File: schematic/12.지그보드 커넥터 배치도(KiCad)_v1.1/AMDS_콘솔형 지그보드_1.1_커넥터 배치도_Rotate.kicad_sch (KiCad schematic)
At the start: 37 parts, among them J1 Fan1, J1C01 POWER, J1C03 TEMP, J1C04 LED_DP1, J1C05 LED_DP2, J1C06 LED_TEMP, J1C07 LED_PSU, J1C08 LED_FAN#1, J1C09 LED_FAN#2, J1C10 DP_USB_SW, J1C15 DP, J1C18 PSU, J1C2 FAN, J2 Fan1, J3 Fan1, J4 Fan1, J5 Fan1, J6 Fan1, P1 Fan1, P2 Fan2, P3 Fan3, P4 Fan4, P5 Fan5, P6 Fan6

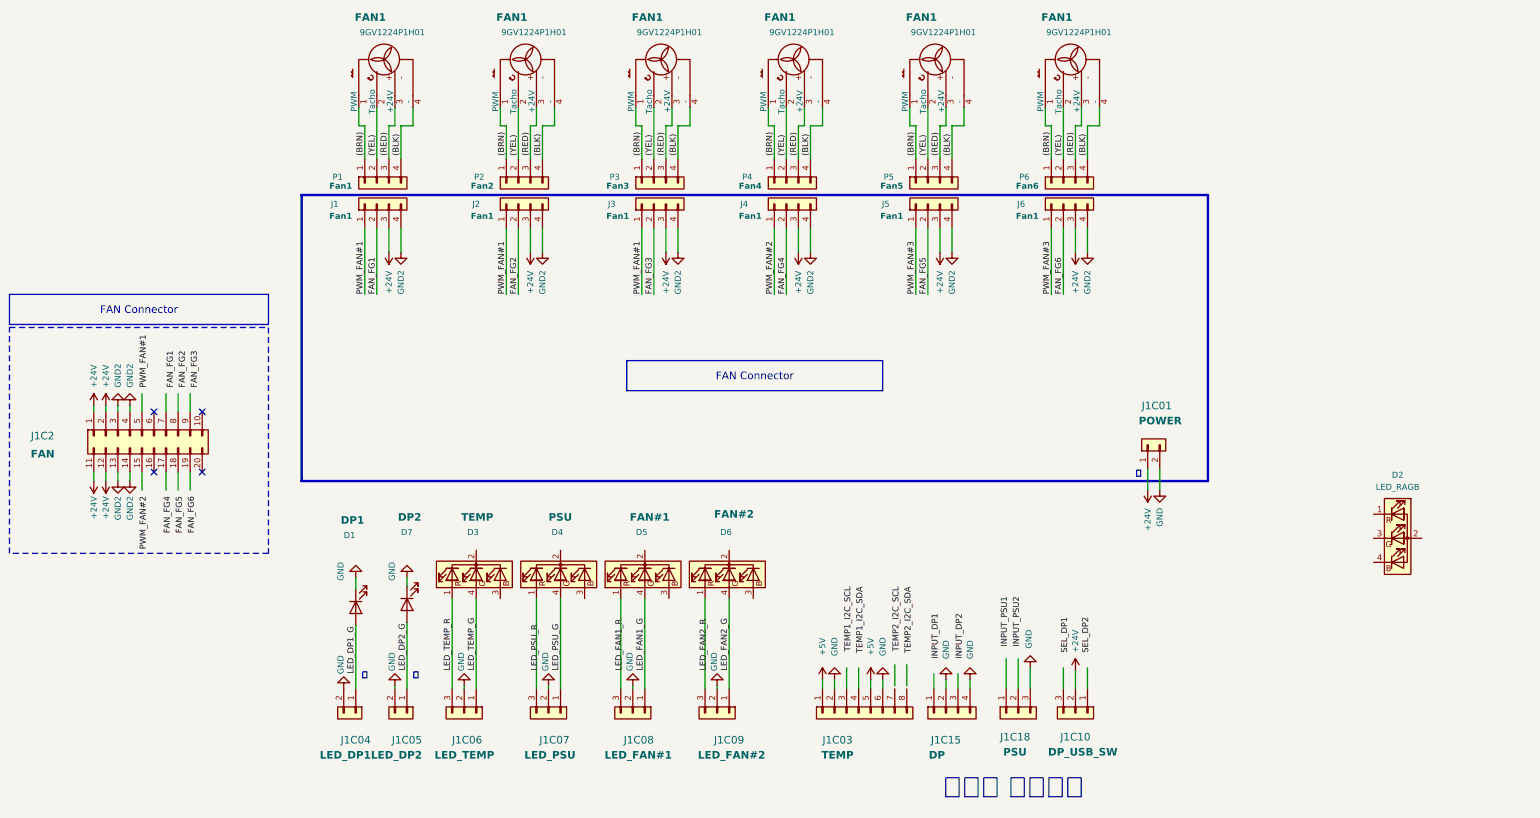
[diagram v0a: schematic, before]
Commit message: 24.12.20B
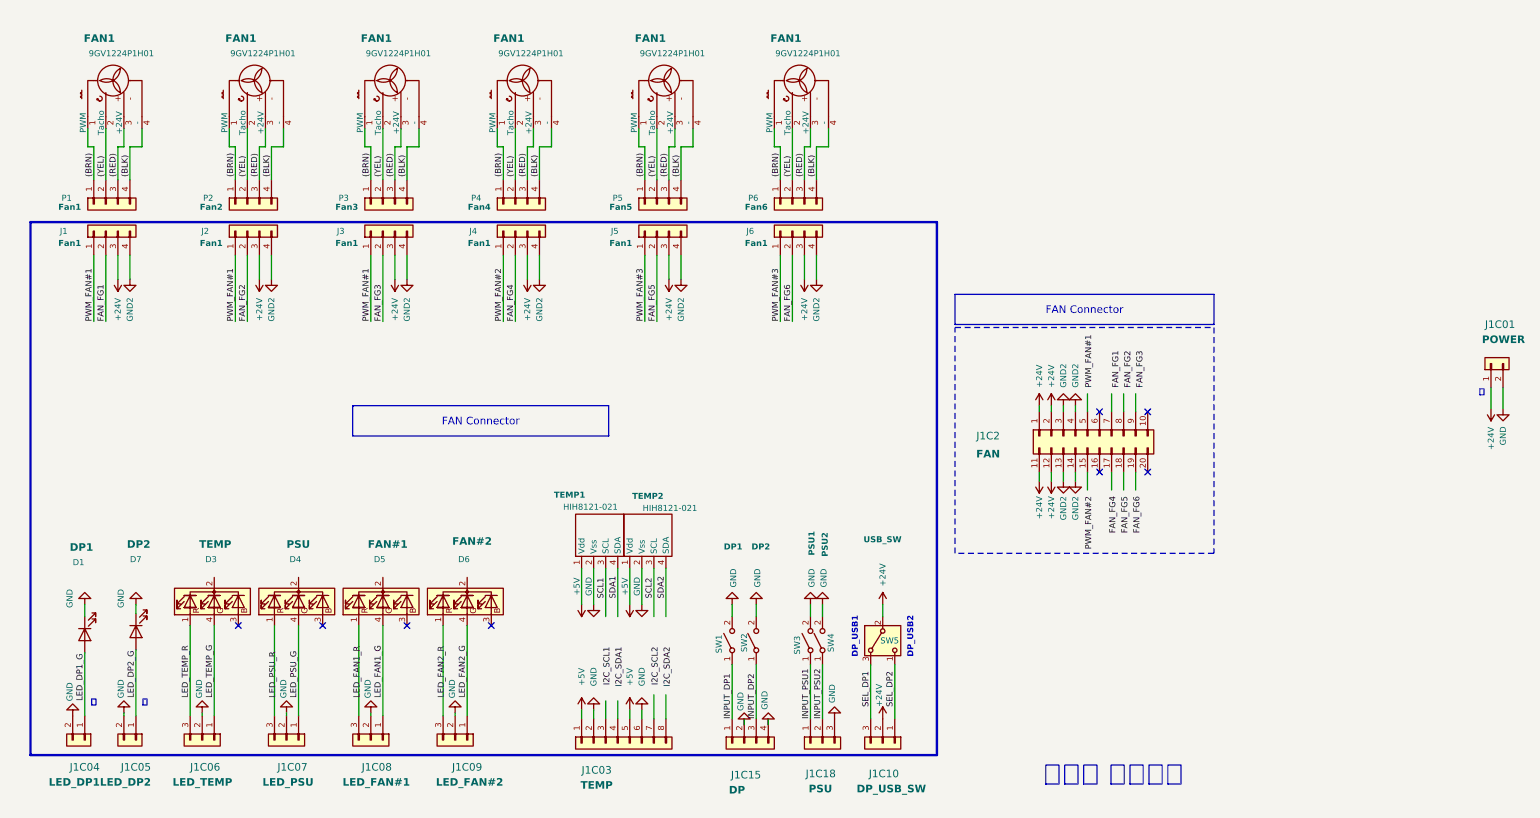
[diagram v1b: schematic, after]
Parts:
- removed D2: LED_RAGB, symbol Device:LED_RAGB
- added SW1: DP1, symbol Switch:SW_SPST
- added SW2: DP2, symbol Switch:SW_SPST
- added SW3: PSU1, symbol Switch:SW_SPST
- added SW4: PSU2, symbol Switch:SW_SPST
- added SW5: USB_SW, symbol Switch:SW_SPDT_321
- added TEMP1, TEMP2: HIH8121-021, symbol Graphic:HIH8121-021
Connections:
- net +24V: now also SW5.2 (B)
- net +5V: now also TEMP1.1 (Vdd), TEMP2.1 (Vdd)
- net GND: now also SW1.2 (B), SW2.2 (B), SW3.2 (B), SW4.2 (B), TEMP1.2 (Vss), TEMP2.2 (Vss)
- net INPUT_DP1: now also J1C15.1 (Pin_1), SW1.1 (A)
- net INPUT_DP2: now also J1C15.3 (Pin_3), SW2.1 (A)
- net INPUT_PSU1: now also J1C18.1 (Pin_1), SW3.1 (A)
- net INPUT_PSU2: now also J1C18.2 (Pin_2), SW4.1 (A)
- net SEL_DP1: now also J1C10.3 (Pin_3), SW5.3 (A)
- net SEL_DP2: now also J1C10.1 (Pin_1), SW5.1 (C)
- new net SCL1: TEMP1.3 (SCL)
- new net SCL2: TEMP2.3 (SCL)
- new net SDA1: TEMP1.4 (SDA)
- new net SDA2: TEMP2.4 (SDA)
- no-connect marks 4 -> 8
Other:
- note added: "DP_USB1"
- note added: "DP_USB2"
- moved on the sheet: D1, D3, D4, D5, D6, D7, FAN1, J1, J1C01, J1C03, J1C04, J1C05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
